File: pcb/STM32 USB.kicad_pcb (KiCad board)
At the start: 2 copper layers, 9 parts, among them U1 STM32L432KBUx

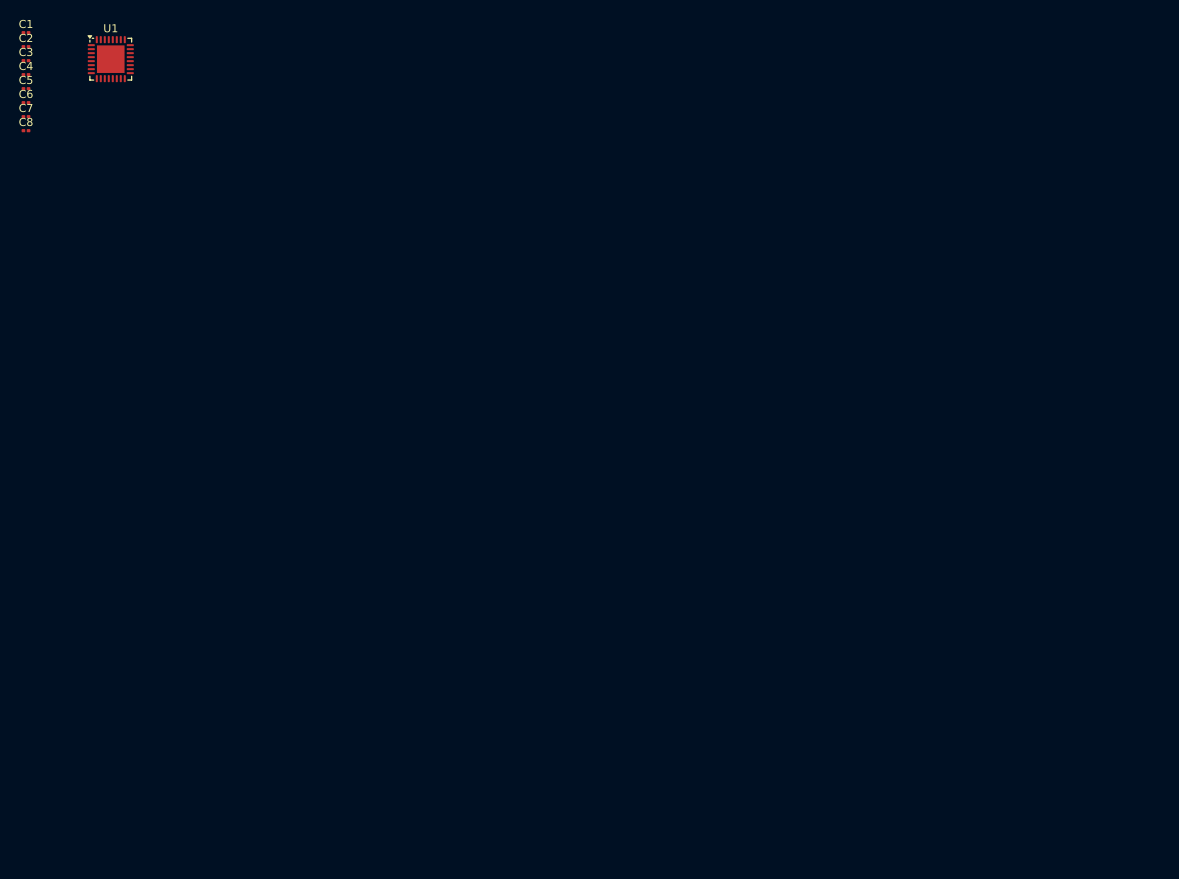
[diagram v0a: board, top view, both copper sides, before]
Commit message: Routed PCB
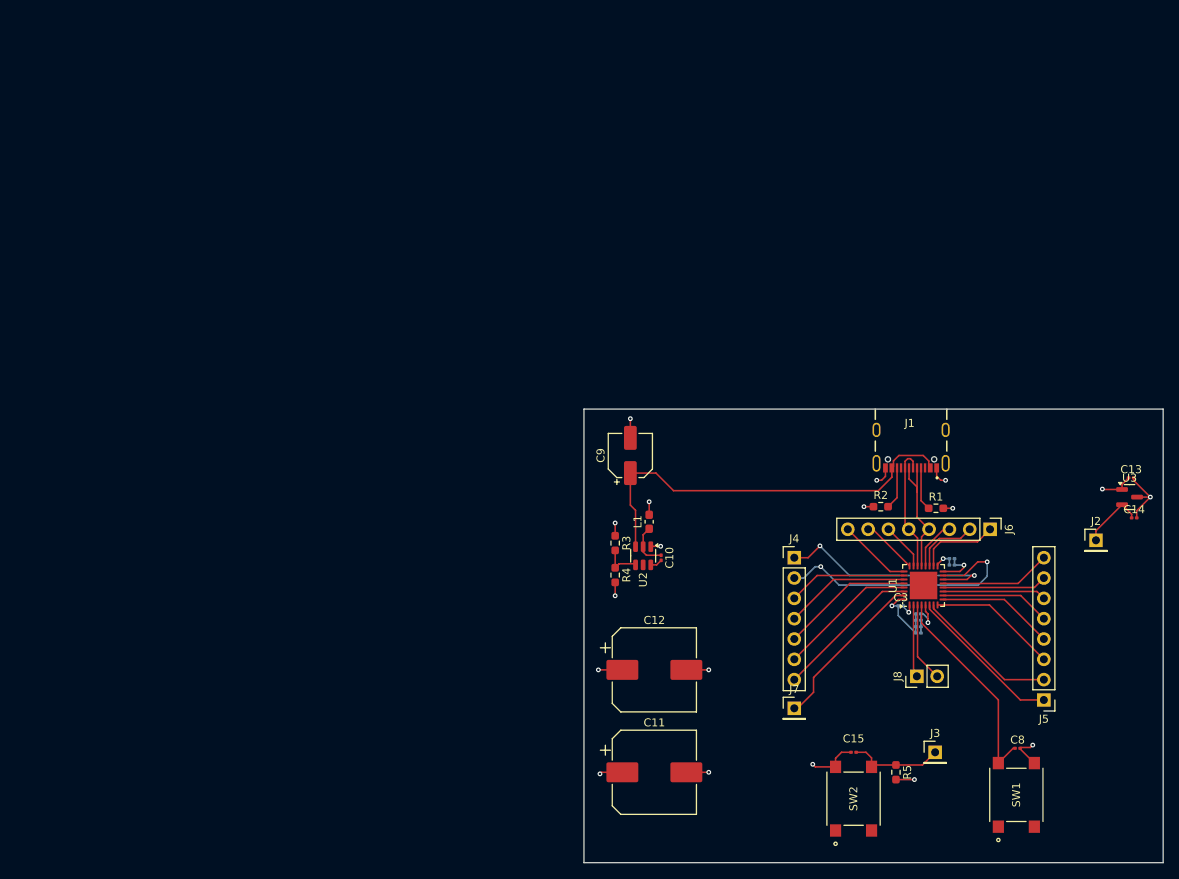
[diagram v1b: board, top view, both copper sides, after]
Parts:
- added C10: 100nF, Capacitor_SMD:C_0201_0603Metric, F.Cu at (122.5, 90.4)
- added C11: 150uF, Capacitor_SMD:CP_Elec_10x10, F.Cu at (121.7, 117.2)
- added C12: 150uF, Capacitor_SMD:CP_Elec_10x10, F.Cu at (121.7, 104.4)
- added C13: 100nF, Capacitor_SMD:C_0201_0603Metric, F.Cu at (181.3, 80.4)
- added C14: 100nF, Capacitor_SMD:C_0201_0603Metric, F.Cu at (181.7, 85.4)
- added C15: 0.1uF, Capacitor_SMD:C_0201_0603Metric, F.Cu at (146.6, 114.7)
- added C9: 10uF, Capacitor_SMD:CP_Elec_5x5.3, F.Cu at (118.7, 77.6)
- added J1: USB4105-GF-A, footprints:GCT_USB4105-GF-A, F.Cu at (153.8, 74.4)
- added J2: Conn_01x01_Pin, Connector_PinHeader_2.54mm:PinHeader_1x01_P2.54mm_Vertical, F.Cu at (176.9, 88.2)
- added J3: Conn_01x01_Pin, Connector_PinHeader_2.54mm:PinHeader_1x01_P2.54mm_Vertical, F.Cu at (156.8, 114.7)
- added J4: Conn_01x07_Pin, Connector_PinHeader_2.54mm:PinHeader_1x07_P2.54mm_Vertical, F.Cu at (139.2, 90.4)
- added J5: Conn_01x08_Pin, Connector_PinHeader_2.54mm:PinHeader_1x08_P2.54mm_Vertical, F.Cu at (170.4, 108.2)
- added J6: Conn_01x08_Pin, Connector_PinHeader_2.54mm:PinHeader_1x08_P2.54mm_Vertical, F.Cu at (163.7, 86.8)
- added J7: Conn_01x01_Pin, Connector_PinHeader_2.54mm:PinHeader_1x01_P2.54mm_Vertical, F.Cu at (139.2, 109.2)
- added J8: Conn_01x02_Pin, Connector_PinHeader_2.54mm:PinHeader_1x02_P2.54mm_Vertical, F.Cu at (154.5, 105.2)
- added L1: 2.2uH, Inductor_SMD:L_0603_1608Metric_Pad1.05x0.95mm_HandSolder, F.Cu at (121.0, 85.9)
- added R1: 5.1k, Resistor_SMD:R_0603_1608Metric_Pad0.98x0.95mm_HandSolder, F.Cu at (156.9, 84.2)
- added R2: 5.1k, Resistor_SMD:R_0603_1608Metric_Pad0.98x0.95mm_HandSolder, F.Cu at (150.0, 84.0)
- added R3: 67k, Resistor_SMD:R_0603_1608Metric_Pad0.98x0.95mm_HandSolder, F.Cu at (116.8, 88.5)
- added R4: 20k, Resistor_SMD:R_0603_1608Metric_Pad0.98x0.95mm_HandSolder, F.Cu at (116.8, 92.5)
- added R5: 10k, Resistor_SMD:R_0603_1608Metric_Pad0.98x0.95mm_HandSolder, F.Cu at (151.9, 117.2)
- added SW1: 222AMVBAR, footprints:222AMVBAR, F.Cu at (166.9, 120.0)
- added SW2: 222AMVBAR, footprints:222AMVBAR, F.Cu at (146.6, 120.5)
- added U2: AP62300TWU, Package_TO_SOT_SMD:TSOT-23-6, F.Cu at (120.3, 90.1)
- added U3: MCP9700Ax-ETT, Package_TO_SOT_SMD:SOT-23, F.Cu at (181.1, 82.8)
- C1, C2, C3, C4, C5, C6, C7: moved to B.Cu
- moved C8 146.0 mm to (167.1, 114.2)
- moved C1 133.1 mm to (158.9, 90.5)
- moved C2 132.6 mm to (158.9, 91.3)
- moved C4 130.3 mm to (154.7, 97.4), turned to 180 degrees
- moved C5 129.8 mm to (154.7, 98.2), turned to 180 degrees
- moved C6 129.4 mm to (154.7, 99.0), turned to 180 degrees
- moved C7 128.9 mm to (154.7, 99.8), turned to 180 degrees
- moved C3 128.8 mm to (152.5, 96.4), turned to 180 degrees
- moved U1 121.0 mm to (155.3, 93.8), turned to 90 degrees
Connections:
- C4 pad 1: +3.3VA -> +3.3V
- C5 pad 1: +3.3VA -> +3.3V
- C6 pad 1: +3.3VA -> +3.3V
- C7 pad 1: +3.3VA -> +3.3V
- U1 pad 10: unconnected-(U1-PA4-Pad10) -> Net-(J5-Pin_5)
- U1 pad 11: unconnected-(U1-PA5-Pad11) -> Net-(J5-Pin_6)
- U1 pad 12: unconnected-(U1-PA6-Pad12) -> Net-(J5-Pin_7)
- U1 pad 13: unconnected-(U1-PA7-Pad13) -> Net-(J5-Pin_8)
- U1 pad 14: unconnected-(U1-PB0-Pad14) -> Net-(J4-Pin_1)
- U1 pad 15: unconnected-(U1-PB1-Pad15) -> Net-(J4-Pin_2)
- U1 pad 18: unconnected-(U1-PA8-Pad18) -> Net-(J6-Pin_1)
- U1 pad 19: unconnected-(U1-PA9-Pad19) -> Net-(J6-Pin_2)
- U1 pad 2: unconnected-(U1-PC14-Pad2) -> Net-(J8-Pin_1)
- U1 pad 20: unconnected-(U1-PA10-Pad20) -> Net-(J6-Pin_3)
- U1 pad 24: unconnected-(U1-PA14-Pad24) -> Net-(J6-Pin_7)
- U1 pad 25: unconnected-(U1-PA15-Pad25) -> Net-(J6-Pin_8)
- U1 pad 26: unconnected-(U1-PB3-Pad26) -> Net-(J4-Pin_3)
- U1 pad 27: unconnected-(U1-PB4-Pad27) -> Net-(J4-Pin_4)
- U1 pad 28: unconnected-(U1-PB5-Pad28) -> Net-(J4-Pin_5)
- U1 pad 29: unconnected-(U1-PB6-Pad29) -> Net-(J4-Pin_6)
- U1 pad 3: unconnected-(U1-PC15-Pad3) -> Net-(J8-Pin_2)
- U1 pad 30: unconnected-(U1-PB7-Pad30) -> Net-(J4-Pin_7)
- U1 pad 31: unconnected-(U1-PH3-Pad31) -> Net-(J7-Pin_1)
- U1 pad 5: +3.3VA -> +3.3V
- U1 pad 6: unconnected-(U1-PA0-Pad6) -> Net-(J5-Pin_1)
- U1 pad 7: unconnected-(U1-PA1-Pad7) -> Net-(J5-Pin_2)
- U1 pad 8: unconnected-(U1-PA2-Pad8) -> Net-(J5-Pin_3)
- U1 pad 9: unconnected-(U1-PA3-Pad9) -> Net-(J5-Pin_4)
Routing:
- net +5V: track 0.00 -> 51.8 mm
- net GND: track 0.00 -> 47.3 mm, vias 0 -> 14
- net Net-(J4-Pin_2): track 0.00 -> 34.1 mm, vias 0 -> 2
- net +3.3V: track 0.00 -> 30.6 mm, vias 0 -> 9
- net Net-(J4-Pin_1): track 0.00 -> 28.8 mm, vias 0 -> 2
- net /NRST: track 0.00 -> 26.6 mm
- net Net-(J7-Pin_1): track 0.00 -> 20.6 mm
- net Net-(J5-Pin_1): track 0.00 -> 19.5 mm
- net Net-(J4-Pin_7): track 0.00 -> 18.3 mm
- net Net-(J5-Pin_2): track 0.00 -> 17.9 mm
- net Net-(J4-Pin_6): track 0.00 -> 17.4 mm
- net /USB_DM: track 0.00 -> 16.7 mm
- net Net-(J4-Pin_5): track 0.00 -> 16.6 mm
- net Net-(J5-Pin_3): track 0.00 -> 16.1 mm
- net /USB_DP: track 0.00 -> 15.8 mm
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- added copper zone on In2.Cu, net +3.3V
- added copper zone on In1.Cu, net GND
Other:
- board outline added: 72.4 x 56.7 mm
- copper layers 2 -> 4
